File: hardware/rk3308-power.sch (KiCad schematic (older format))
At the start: 25 parts, among them Q110 LN235N3T5G, U100 RK3308, Y100 24MHz,12pF,10ppm

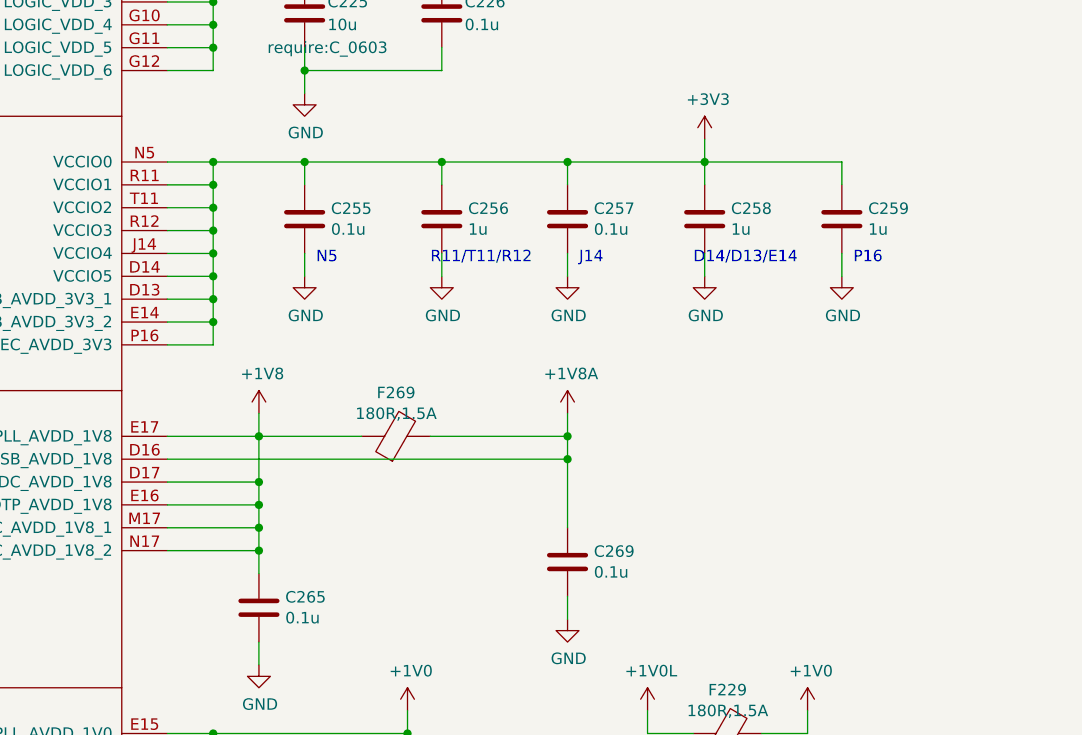
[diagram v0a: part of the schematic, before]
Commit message: wip
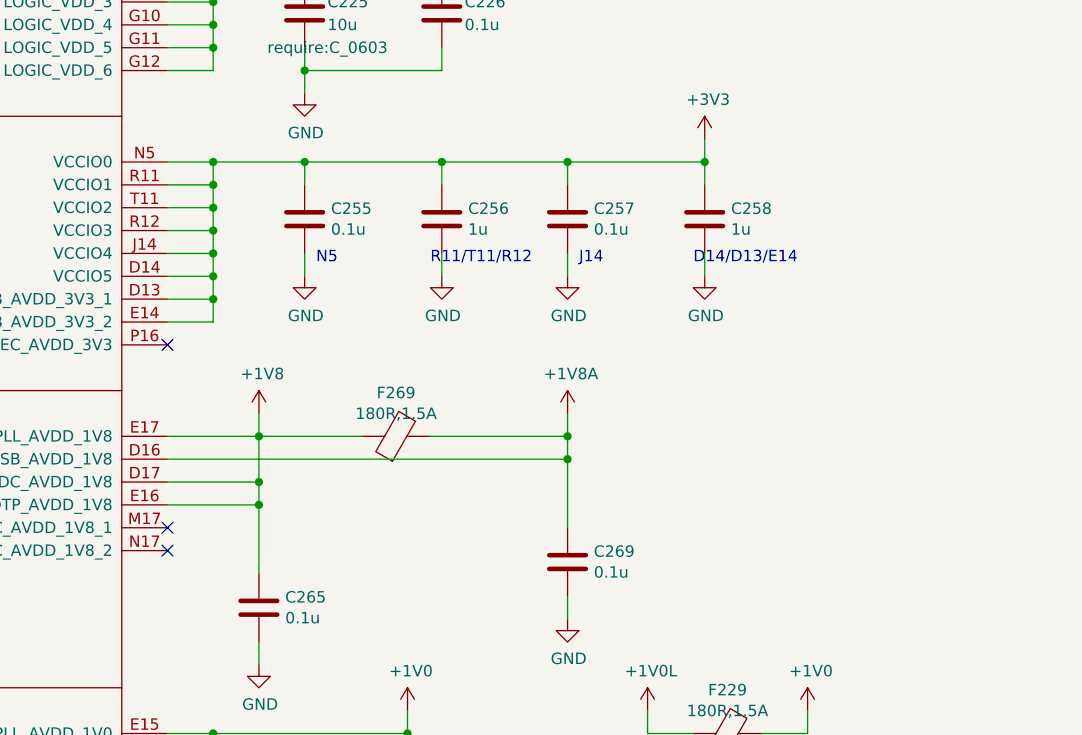
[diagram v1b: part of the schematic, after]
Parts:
- removed C259: 1u, require:C_0402, symbol Device:C
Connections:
- net +1V8: no longer U100.M17 (CODEC_AVDD_1V8_1), U100.N17 (CODEC_AVDD_1V8_2)
- net +3V3: no longer U100.P16 (CODEC_AVDD_3V3)
- no-connect marks 1 -> 4
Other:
- note removed: "P16"
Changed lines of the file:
@@
 	3300 5550 3300 5450
 Connection ~ 3300 5450
-Wire Wire Line
-	3100 5650 3300 5650
-Wire Wire Line
-	3300 5650 3300 5550
-Connection ~ 3300 5550
 $Comp
 L Device:C C?
@@
 Wire Wire Line
 	4850 6150 4850 6450
-Wire Wire Line
-	3500 6350 3500 6450
-Wire Wire Line
-	3100 6450 3500 6450
-Connection ~ 3500 6450
-Wire Wire Line
-	3500 6450 3500 6550
-Wire Wire Line
-	3100 6550 3500 6550
-Connection ~ 3500 6550
-Wire Wire Line
-	3500 6550 3500 6650
 Wire Wire Line
 	3100 8050 3300 8050
@@
 Text Notes 5400 5300 0    50   ~ 0
 D14/D13/E14
-$Comp
-L Device:C C?
-U 1 1 5C781190
-P 6050 5100
-AR Path="/5CED3BD3/5C781190" Ref="C?"  Part="1"
-AR Path="/5C325762/5C781190" Ref="C259"  Part="1"
-F 0 "C259" H 6165 5146 50  0000 L CNN
-F 1 "1u" H 6165 5055 50  0000 L CNN
-F 2 "require:C_0402" H 6088 4950 50  0001 C CNN
-F 3 "~" H 6050 5100 50  0001 C CNN
-	1    6050 5100
-	1    0    0    -1
-$EndComp
-Wire Wire Line
-	5450 4850 6050 4850
-Wire Wire Line
-	6050 4850 6050 4950
-$Comp
-L power:GND #PWR?
-U 1 1 5C7ABB6E
-P 6050 5350
-AR Path="/5CED3BD3/5C7ABB6E" Ref="#PWR?"  Part="1"
-AR Path="/5C325762/5C7ABB6E" Ref="#PWR0110"  Part="1"
-F 0 "#PWR0110" H 6050 5100 50  0001 C CNN
-F 1 "GND" H 6055 5177 50  0000 C CNN
-F 2 "" H 6050 5350 50  0001 C CNN
-F 3 "" H 6050 5350 50  0001 C CNN
-	1    6050 5350
-	1    0    0    -1
-$EndComp
-Wire Wire Line
-	6050 5250 6050 5350
-Text Notes 6100 5300 0    50   ~ 0
-P16
+NoConn ~ 3100 5650
+Wire Wire Line
+	3500 6350 3500 6650
+NoConn ~ 3100 6450
+NoConn ~ 3100 6550
 $EndSCHEMATC

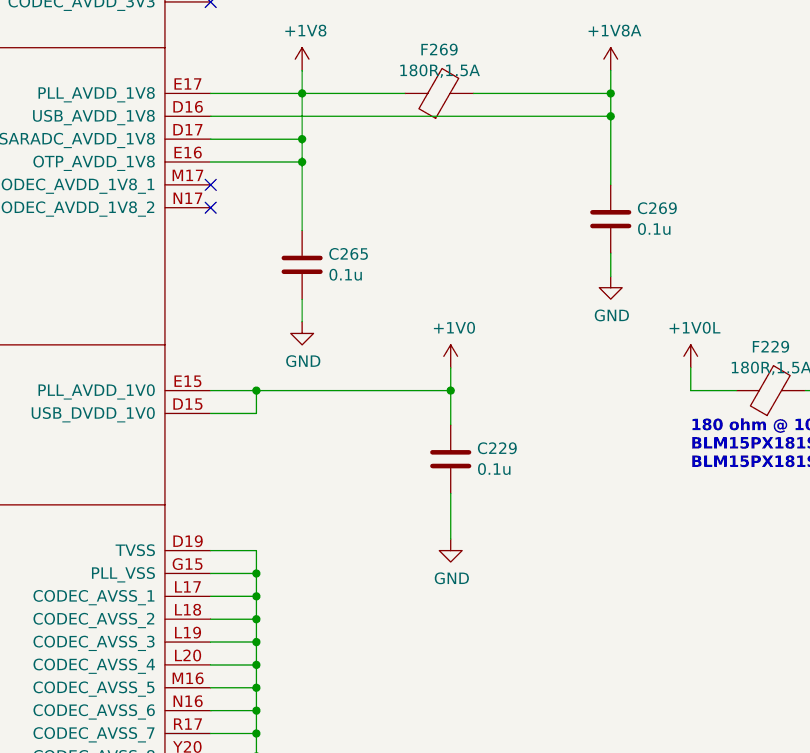
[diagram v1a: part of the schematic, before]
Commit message: wip
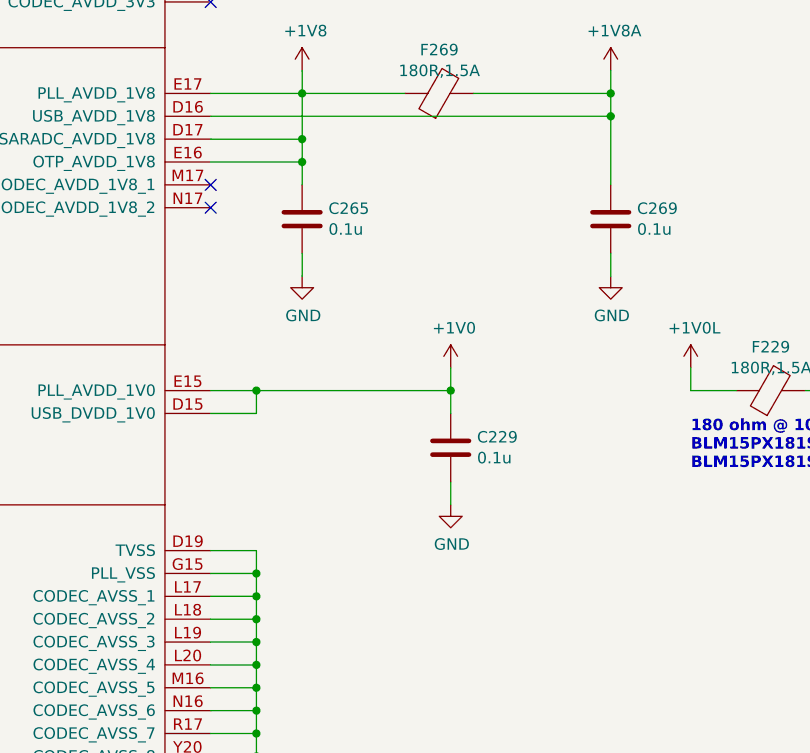
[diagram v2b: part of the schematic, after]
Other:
- moved on the sheet: C229, C265
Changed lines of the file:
@@
 L Device:C C229
 U 1 1 5C84BC04
-P 4150 7650
-F 0 "C229" H 4265 7696 50  0000 L CNN
-F 1 "0.1u" H 4265 7605 50  0000 L CNN
-F 2 "require:C_0402" H 4188 7500 50  0001 C CNN
-F 3 "~" H 4150 7650 50  0001 C CNN
-	1    4150 7650
-	1    0    0    -1
-$EndComp
-Wire Wire Line
-	4150 7800 4150 8000
+P 4150 7600
+F 0 "C229" H 4265 7646 50  0000 L CNN
+F 1 "0.1u" H 4265 7555 50  0000 L CNN
+F 2 "require:C_0402" H 4188 7450 50  0001 C CNN
+F 3 "~" H 4150 7600 50  0001 C CNN
+	1    4150 7600
+	1    0    0    -1
+$EndComp
+Wire Wire Line
+	4150 7750 4150 7850
 $Comp
 L power:GND #PWR0203
 U 1 1 5C9782CF
-P 4150 8000
-F 0 "#PWR0203" H 4150 7750 50  0001 C CNN
-F 1 "GND" H 4155 7827 50  0000 C CNN
-F 2 "" H 4150 8000 50  0001 C CNN
-F 3 "" H 4150 8000 50  0001 C CNN
-	1    4150 8000
+P 4150 7850
+F 0 "#PWR0203" H 4150 7600 50  0001 C CNN
+F 1 "GND" H 4155 7677 50  0000 C CNN
+F 2 "" H 4150 7850 50  0001 C CNN
+F 3 "" H 4150 7850 50  0001 C CNN
+	1    4150 7850
 	1    0    0    -1
 $EndComp
@@
 L Device:C C265
 U 1 1 5C9A47A9
-P 3500 6800
-F 0 "C265" H 3615 6846 50  0000 L CNN
-F 1 "0.1u" H 3615 6755 50  0000 L CNN
-F 2 "require:C_0402" H 3538 6650 50  0001 C CNN
-F 3 "~" H 3500 6800 50  0001 C CNN
-	1    3500 6800
+P 3500 6600
+F 0 "C265" H 3615 6646 50  0000 L CNN
+F 1 "0.1u" H 3615 6555 50  0000 L CNN
+F 2 "require:C_0402" H 3538 6450 50  0001 C CNN
+F 3 "~" H 3500 6600 50  0001 C CNN
+	1    3500 6600
 	1    0    0    -1
 $EndComp
@@
 L power:GND #PWR0205
 U 1 1 5C9FD96A
-P 3500 7050
-F 0 "#PWR0205" H 3500 6800 50  0001 C CNN
-F 1 "GND" H 3505 6877 50  0000 C CNN
-F 2 "" H 3500 7050 50  0001 C CNN
-F 3 "" H 3500 7050 50  0001 C CNN
-	1    3500 7050
+P 3500 6850
+F 0 "#PWR0205" H 3500 6600 50  0001 C CNN
+F 1 "GND" H 3505 6677 50  0000 C CNN
+F 2 "" H 3500 6850 50  0001 C CNN
+F 3 "" H 3500 6850 50  0001 C CNN
+	1    3500 6850
 	1    0    0    -1
 $EndComp
@@
 Connection ~ 4850 6150
 Wire Wire Line
-	3500 6950 3500 7050
+	3500 6750 3500 6850
 Wire Wire Line
 	3100 6250 3500 6250
@@
 Connection ~ 4150 7350
 Wire Wire Line
-	4150 7350 4150 7500
+	4150 7350 4150 7450
 Wire Wire Line
 	3100 7450 3300 7450
@@
 NoConn ~ 3100 5650
 Wire Wire Line
-	3500 6350 3500 6650
+	3500 6350 3500 6450
 NoConn ~ 3100 6450
 NoConn ~ 3100 6550
